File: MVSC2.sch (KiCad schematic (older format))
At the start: 172 parts, among them J1 USB_C-SIGNAL, J16 ADC_HB, J17 ESTP0, J18 ESTP1, J19 ESTP2, J2 SWD, J20 ESTP3, J21 ESTP4, J22 ESTP5, J23 POWER, J29 ADC_E, J3 EXPP0, J30 HSES, J31 HSES, J32 HSES, J4 EXPP1, J6 PWM_E, J7 PWM_HB, J9 PWM_FAN, P1 STP0, P2 STP2, P3 STP4, P4 STP1, P5 STP3, P6 STP5, Q1 AO3400A, Q10 AO3400A, Q2 AO3400A, Q3 AO3400A, Q4 AO3400A, Q5 AO3400A, Q6 AO3400A, SW1 SKRKAEE020, SW2 SKRKAEE020, U1 XC6206P332MR, U10 TMC2208-LA-T, U11 TMC2208-LA-T, U12 TMC2208-LA-T, U3 STM32F411CEU6, U4 CH912LSR, U5 TMC2208-LA-T, U6 TMC2208-LA-T, U7 TMC2208-LA-T, U8 CH912LSR, U9 CH912LSR, Y1 25MHZ 12pF, Y2 32.768KHz 12.5pF

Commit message: working version with mosfets
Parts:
- J1: LCSC (none) -> C165948
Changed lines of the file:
@@
 F 2 "Connector_USB:USB_C_Receptacle_HRO_TYPE-C-31-M-12" H 2000 3400 50  0001 C CNN
 F 3 "https://www.usb.org/sites/default/files/documents/usb_type-c.zip" H 2000 3400 50  0001 C CNN
+F 4 "C165948" H 1850 3400 50  0001 C CNN "LCSC"
 	1    1850 3400
 	1    0    0    -1

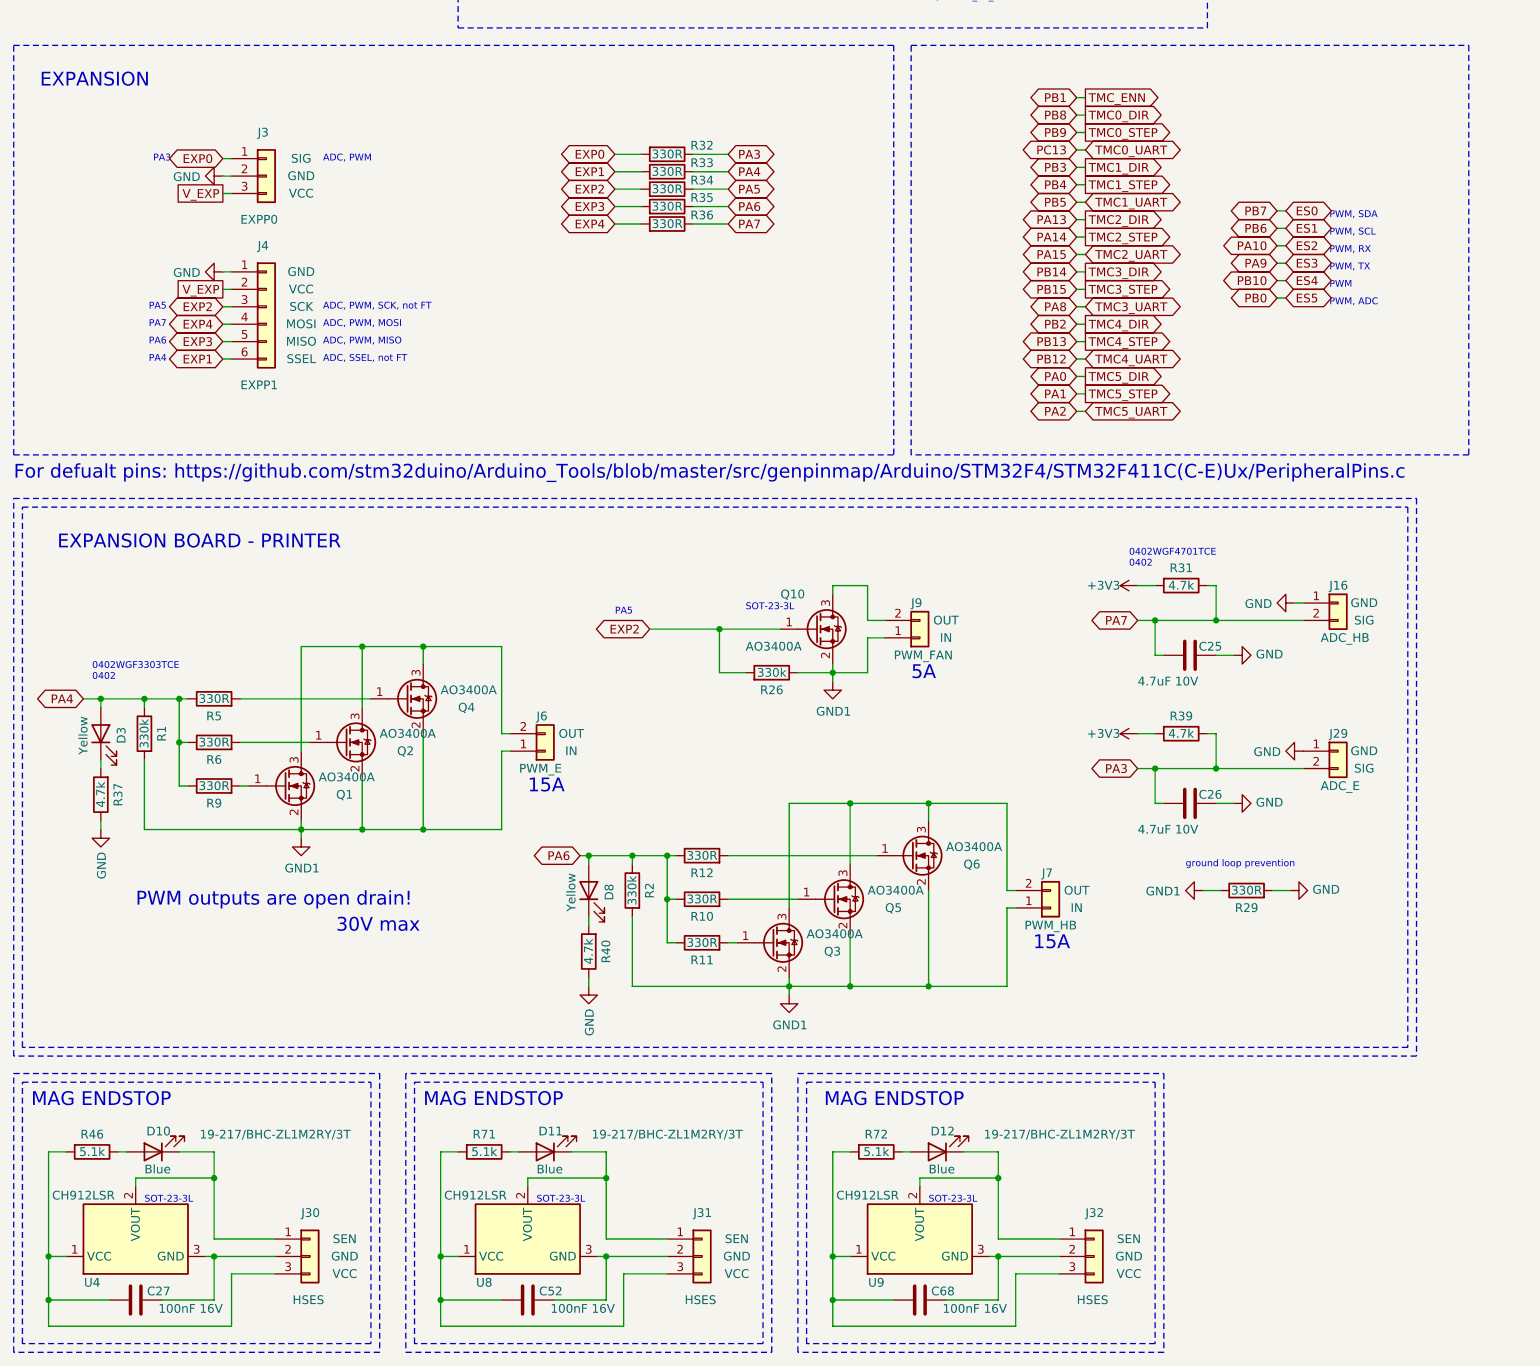
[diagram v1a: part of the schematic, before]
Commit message: final, ordered
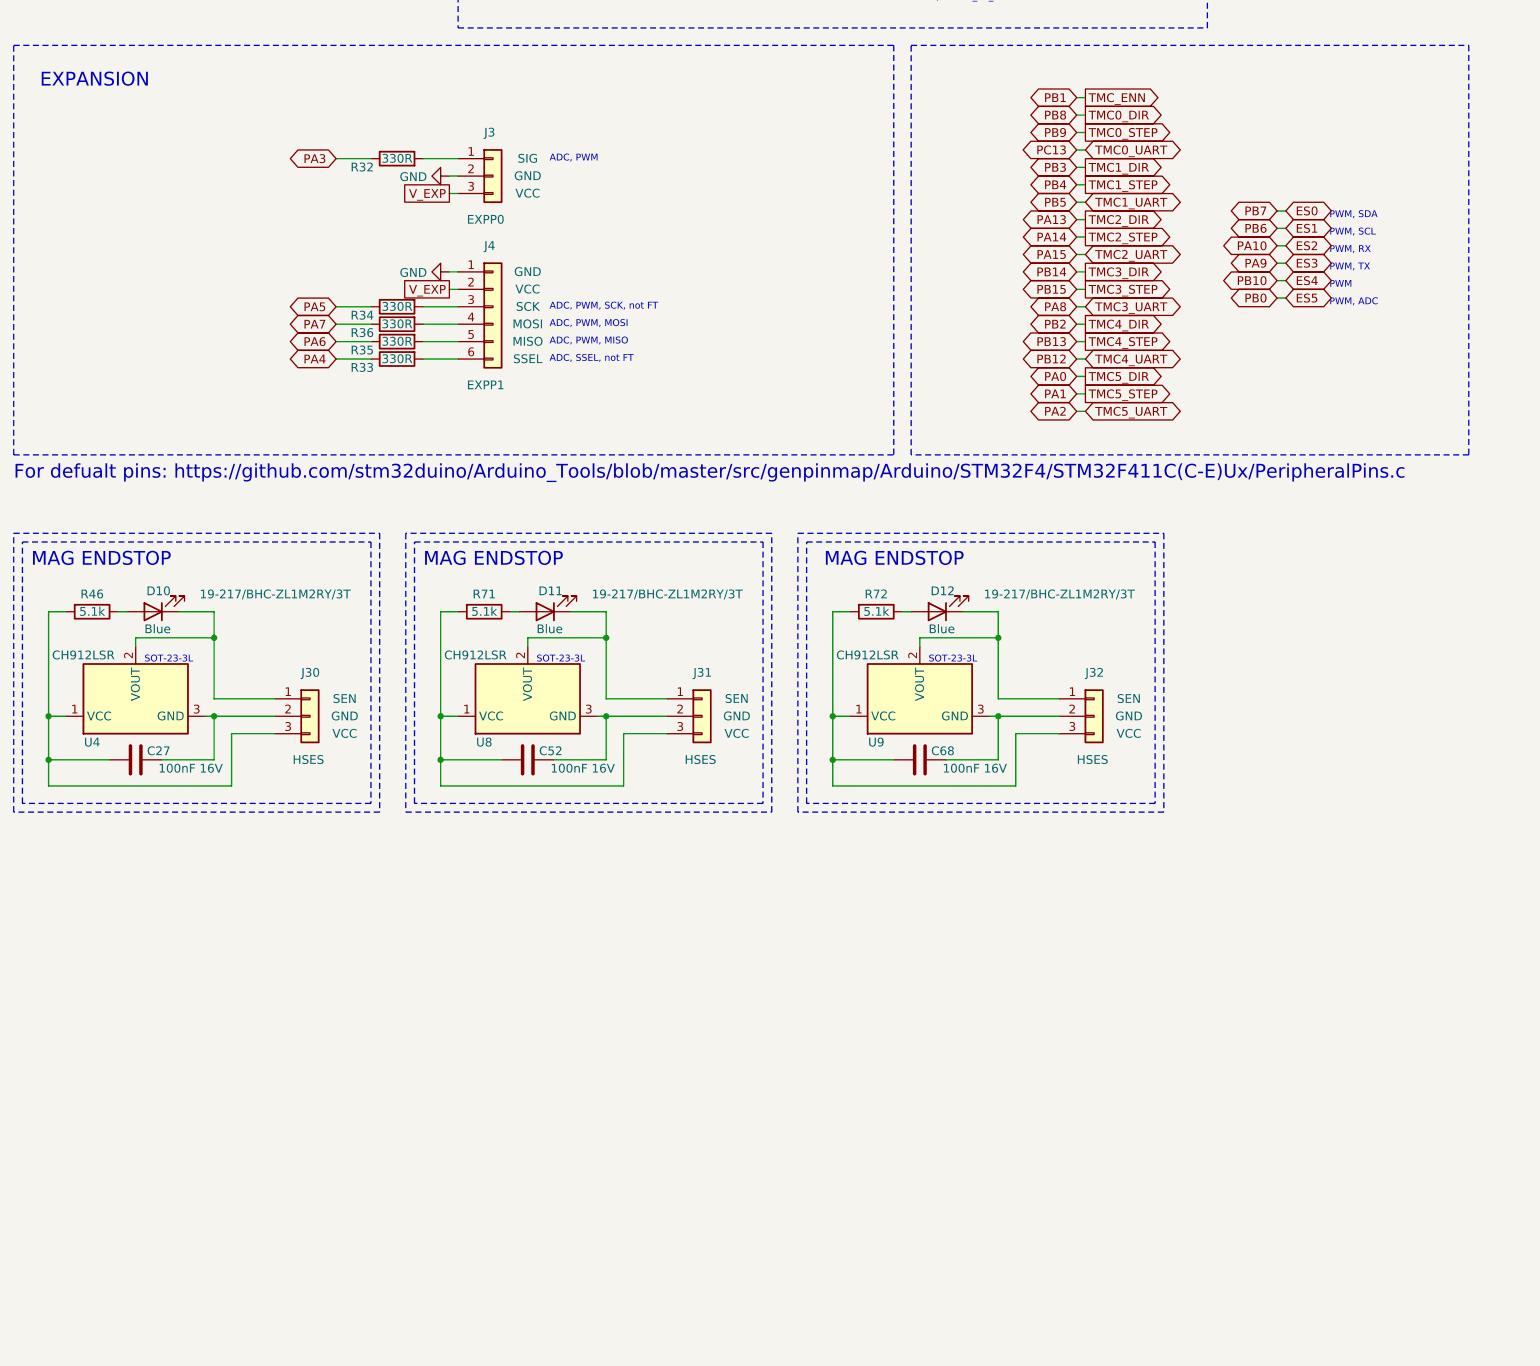
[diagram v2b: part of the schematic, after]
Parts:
- removed C25, C26: 4.7uF 10V, Capacitor_SMD:C_0402_1005Metric, symbol Device:C
- removed D3, D8: Yellow, LED_SMD:LED_0603_1608Metric, symbol Device:LED
- removed J16: ADC_HB, Connector_JST:JST_PH_B2B-PH-K_1x02_P2.00mm_Vertical, symbol Connector_Generic:Conn_01x02
- removed J29: ADC_E, Connector_JST:JST_PH_B2B-PH-K_1x02_P2.00mm_Vertical, symbol Connector_Generic:Conn_01x02
- removed J6: PWM_E, Connector_AMASS:AMASS_XT30U-F_1x02_P5.0mm_Vertical, symbol Connector_Generic:Conn_01x02
- removed J7: PWM_HB, Connector_AMASS:AMASS_XT30U-F_1x02_P5.0mm_Vertical, symbol Connector_Generic:Conn_01x02
- removed J9: PWM_FAN, Connector_JST:JST_PH_B2B-PH-K_1x02_P2.00mm_Vertical, symbol Connector_Generic:Conn_01x02
- removed Q1, Q10, Q2, Q3, Q4, Q5, Q6: AO3400A, Package_TO_SOT_SMD:SOT-23W, symbol Transistor_FET:2N7002
- removed R1, R2, R26: 330k, Resistor_SMD:R_0402_1005Metric, symbol Device:R
- removed R10, R11, R12, R29, R5, R6, R9: 330R, Resistor_SMD:R_0402_1005Metric, symbol Device:R
- removed R31, R37, R39, R40: 4.7k, Resistor_SMD:R_0402_1005Metric, symbol Device:R
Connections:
- net EXP0: no longer names the net of J3.1 (Pin_1), R32.2
- net EXP1: no longer names the net of J4.6 (Pin_6), R33.2
- net EXP2: no longer names the net of J4.3 (Pin_3), R34.2
- net EXP3: no longer names the net of J4.5 (Pin_5), R35.2
- net EXP4: no longer names the net of J4.4 (Pin_4), R36.2
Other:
- note removed: "0402WGF3303TCE\n0402"
- note removed: "0402WGF4701TCE\n0402"
- note removed: "15A"
- note removed: "30V max"
- note removed: "5A"
- note removed: "EXPANSION BOARD - PRINTER"
- note removed: "PA3"
- note removed: "PA4"
- note removed: "PA5"
- note removed: "PA6"
- note removed: "PA7"
- note removed: "PWM outputs are open drain!"
- note removed: "ground loop prevention"
- moved on the sheet: C27, C52, C68, D10, D11, D12, J3, J30, J31, J32, J4, R32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
